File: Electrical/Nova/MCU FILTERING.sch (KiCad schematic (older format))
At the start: 13 parts

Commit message: Added Barometer, Flash, SD, and Power Supply
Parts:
- C? (x13): symbol Nova_Microcontroller:C -> Nova-rescue:C-Nova_Microcontroller
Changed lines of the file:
@@
 $Descr A4 11693 8268
 encoding utf-8
-Sheet 7 9
+Sheet 7 13
 Title "Microcontroller"
 Date "2020-07-02"
@@
 $EndBitmap
 $Comp
-L Nova_Microcontroller:C C?
+L Nova-rescue:C-Nova_Microcontroller C?
 U 1 1 5EEB15D0
 P 1600 3450
@@
 $EndComp
 $Comp
-L Nova_Microcontroller:C C?
+L Nova-rescue:C-Nova_Microcontroller C?
 U 1 1 5EEA7BC1
 P 2150 3450
@@
 $EndComp
 $Comp
-L Nova_Microcontroller:C C?
+L Nova-rescue:C-Nova_Microcontroller C?
 U 1 1 5EEA7EAA
 P 2650 3450
@@
 $EndComp
 $Comp
-L Nova_Microcontroller:C C?
+L Nova-rescue:C-Nova_Microcontroller C?
 U 1 1 5EEA8258
 P 3150 3450
@@
 $EndComp
 $Comp
-L Nova_Microcontroller:C C?
+L Nova-rescue:C-Nova_Microcontroller C?
 U 1 1 5EEA85B4
 P 3650 3450
@@
 $EndComp
 $Comp
-L Nova_Microcontroller:C C?
+L Nova-rescue:C-Nova_Microcontroller C?
 U 1 1 5EEA893A
 P 4150 3450
@@
 	3650 3000 4150 3000
 $Comp
-L Nova_Microcontroller:C C?
+L Nova-rescue:C-Nova_Microcontroller C?
 U 1 1 5EEADB63
 P 6350 3450
@@
 	6350 3300 6350 3100
 $Comp
-L Nova_Microcontroller:C C?
+L Nova-rescue:C-Nova_Microcontroller C?
 U 1 1 5EEAF36F
 P 4900 3450
@@
 $EndComp
 $Comp
-L Nova_Microcontroller:C C?
+L Nova-rescue:C-Nova_Microcontroller C?
 U 1 1 5EEAF915
 P 5450 3450
@@
 	5150 3100 5450 3100
 $Comp
-L Nova_Microcontroller:C C?
+L Nova-rescue:C-Nova_Microcontroller C?
 U 1 1 5EEB4CA7
 P 7350 3450
@@
 $EndComp
 $Comp
-L Nova_Microcontroller:C C?
+L Nova-rescue:C-Nova_Microcontroller C?
 U 1 1 5EEB51E9
 P 8000 3450
@@
 VREF CAPS
 $Comp
-L Nova_Microcontroller:C C?
+L Nova-rescue:C-Nova_Microcontroller C?
 U 1 1 5EEBBE66
 P 9450 3450
@@
 $EndComp
 $Comp
-L Nova_Microcontroller:C C?
+L Nova-rescue:C-Nova_Microcontroller C?
 U 1 1 5EEBC1C7
 P 10050 3450

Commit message: Fixed Power Supply
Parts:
- C? (x13): symbol Nova-rescue:C-Nova_Microcontroller -> Nova-rescue:C-Nova_Microcontroller-Nova-rescue
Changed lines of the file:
@@
 $EndBitmap
 $Comp
-L Nova-rescue:C-Nova_Microcontroller C?
+L Nova-rescue:C-Nova_Microcontroller-Nova-rescue C?
 U 1 1 5EEB15D0
 P 1600 3450
@@
 $EndComp
 $Comp
-L Nova-rescue:C-Nova_Microcontroller C?
+L Nova-rescue:C-Nova_Microcontroller-Nova-rescue C?
 U 1 1 5EEA7BC1
 P 2150 3450
@@
 $EndComp
 $Comp
-L Nova-rescue:C-Nova_Microcontroller C?
+L Nova-rescue:C-Nova_Microcontroller-Nova-rescue C?
 U 1 1 5EEA7EAA
 P 2650 3450
@@
 $EndComp
 $Comp
-L Nova-rescue:C-Nova_Microcontroller C?
+L Nova-rescue:C-Nova_Microcontroller-Nova-rescue C?
 U 1 1 5EEA8258
 P 3150 3450
@@
 $EndComp
 $Comp
-L Nova-rescue:C-Nova_Microcontroller C?
+L Nova-rescue:C-Nova_Microcontroller-Nova-rescue C?
 U 1 1 5EEA85B4
 P 3650 3450
@@
 $EndComp
 $Comp
-L Nova-rescue:C-Nova_Microcontroller C?
+L Nova-rescue:C-Nova_Microcontroller-Nova-rescue C?
 U 1 1 5EEA893A
 P 4150 3450
@@
 	3650 3000 4150 3000
 $Comp
-L Nova-rescue:C-Nova_Microcontroller C?
+L Nova-rescue:C-Nova_Microcontroller-Nova-rescue C?
 U 1 1 5EEADB63
 P 6350 3450
@@
 	6350 3300 6350 3100
 $Comp
-L Nova-rescue:C-Nova_Microcontroller C?
+L Nova-rescue:C-Nova_Microcontroller-Nova-rescue C?
 U 1 1 5EEAF36F
 P 4900 3450
@@
 $EndComp
 $Comp
-L Nova-rescue:C-Nova_Microcontroller C?
+L Nova-rescue:C-Nova_Microcontroller-Nova-rescue C?
 U 1 1 5EEAF915
 P 5450 3450
@@
 	5150 3100 5450 3100
 $Comp
-L Nova-rescue:C-Nova_Microcontroller C?
+L Nova-rescue:C-Nova_Microcontroller-Nova-rescue C?
 U 1 1 5EEB4CA7
 P 7350 3450
@@
 $EndComp
 $Comp
-L Nova-rescue:C-Nova_Microcontroller C?
+L Nova-rescue:C-Nova_Microcontroller-Nova-rescue C?
 U 1 1 5EEB51E9
 P 8000 3450
@@
 VREF CAPS
 $Comp
-L Nova-rescue:C-Nova_Microcontroller C?
+L Nova-rescue:C-Nova_Microcontroller-Nova-rescue C?
 U 1 1 5EEBBE66
 P 9450 3450
@@
 $EndComp
 $Comp
-L Nova-rescue:C-Nova_Microcontroller C?
+L Nova-rescue:C-Nova_Microcontroller-Nova-rescue C?
 U 1 1 5EEBC1C7
 P 10050 3450

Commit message: Added Gyroscope
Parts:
- C? (x13): symbol Nova-rescue:C-Nova_Microcontroller-Nova-rescue -> Nova-rescue:C-Nova_Microcontroller-Nova-rescue-Nova-rescue
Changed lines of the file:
@@
 $Descr A4 11693 8268
 encoding utf-8
-Sheet 7 13
+Sheet 7 14
 Title "Microcontroller"
 Date "2020-07-02"
@@
 $EndBitmap
 $Comp
-L Nova-rescue:C-Nova_Microcontroller-Nova-rescue C?
+L Nova-rescue:C-Nova_Microcontroller-Nova-rescue-Nova-rescue C?
 U 1 1 5EEB15D0
 P 1600 3450
@@
 $EndComp
 $Comp
-L Nova-rescue:C-Nova_Microcontroller-Nova-rescue C?
+L Nova-rescue:C-Nova_Microcontroller-Nova-rescue-Nova-rescue C?
 U 1 1 5EEA7BC1
 P 2150 3450
@@
 $EndComp
 $Comp
-L Nova-rescue:C-Nova_Microcontroller-Nova-rescue C?
+L Nova-rescue:C-Nova_Microcontroller-Nova-rescue-Nova-rescue C?
 U 1 1 5EEA7EAA
 P 2650 3450
@@
 $EndComp
 $Comp
-L Nova-rescue:C-Nova_Microcontroller-Nova-rescue C?
+L Nova-rescue:C-Nova_Microcontroller-Nova-rescue-Nova-rescue C?
 U 1 1 5EEA8258
 P 3150 3450
@@
 $EndComp
 $Comp
-L Nova-rescue:C-Nova_Microcontroller-Nova-rescue C?
+L Nova-rescue:C-Nova_Microcontroller-Nova-rescue-Nova-rescue C?
 U 1 1 5EEA85B4
 P 3650 3450
@@
 $EndComp
 $Comp
-L Nova-rescue:C-Nova_Microcontroller-Nova-rescue C?
+L Nova-rescue:C-Nova_Microcontroller-Nova-rescue-Nova-rescue C?
 U 1 1 5EEA893A
 P 4150 3450
@@
 	3650 3000 4150 3000
 $Comp
-L Nova-rescue:C-Nova_Microcontroller-Nova-rescue C?
+L Nova-rescue:C-Nova_Microcontroller-Nova-rescue-Nova-rescue C?
 U 1 1 5EEADB63
 P 6350 3450
@@
 	6350 3300 6350 3100
 $Comp
-L Nova-rescue:C-Nova_Microcontroller-Nova-rescue C?
+L Nova-rescue:C-Nova_Microcontroller-Nova-rescue-Nova-rescue C?
 U 1 1 5EEAF36F
 P 4900 3450
@@
 $EndComp
 $Comp
-L Nova-rescue:C-Nova_Microcontroller-Nova-rescue C?
+L Nova-rescue:C-Nova_Microcontroller-Nova-rescue-Nova-rescue C?
 U 1 1 5EEAF915
 P 5450 3450
@@
 	5150 3100 5450 3100
 $Comp
-L Nova-rescue:C-Nova_Microcontroller-Nova-rescue C?
+L Nova-rescue:C-Nova_Microcontroller-Nova-rescue-Nova-rescue C?
 U 1 1 5EEB4CA7
 P 7350 3450
@@
 $EndComp
 $Comp
-L Nova-rescue:C-Nova_Microcontroller-Nova-rescue C?
+L Nova-rescue:C-Nova_Microcontroller-Nova-rescue-Nova-rescue C?
 U 1 1 5EEB51E9
 P 8000 3450
@@
 VREF CAPS
 $Comp
-L Nova-rescue:C-Nova_Microcontroller-Nova-rescue C?
+L Nova-rescue:C-Nova_Microcontroller-Nova-rescue-Nova-rescue C?
 U 1 1 5EEBBE66
 P 9450 3450
@@
 $EndComp
 $Comp
-L Nova-rescue:C-Nova_Microcontroller-Nova-rescue C?
+L Nova-rescue:C-Nova_Microcontroller-Nova-rescue-Nova-rescue C?
 U 1 1 5EEBC1C7
 P 10050 3450

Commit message: Added Gyro pins. Organized Schematic
Need to determine if we need the interrupt pins for the sensors.
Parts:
- C? (x13): symbol Nova-rescue:C-Nova_Microcontroller-Nova-rescue-Nova-rescue -> Nova-rescue:C-Nova_Microcontroller-Nova-rescue-Nova-rescue-Nova-rescue
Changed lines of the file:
@@
 $EndBitmap
 $Comp
-L Nova-rescue:C-Nova_Microcontroller-Nova-rescue-Nova-rescue C?
+L Nova-rescue:C-Nova_Microcontroller-Nova-rescue-Nova-rescue-Nova-rescue C?
 U 1 1 5EEB15D0
 P 1600 3450
@@
 $EndComp
 $Comp
-L Nova-rescue:C-Nova_Microcontroller-Nova-rescue-Nova-rescue C?
+L Nova-rescue:C-Nova_Microcontroller-Nova-rescue-Nova-rescue-Nova-rescue C?
 U 1 1 5EEA7BC1
 P 2150 3450
@@
 $EndComp
 $Comp
-L Nova-rescue:C-Nova_Microcontroller-Nova-rescue-Nova-rescue C?
+L Nova-rescue:C-Nova_Microcontroller-Nova-rescue-Nova-rescue-Nova-rescue C?
 U 1 1 5EEA7EAA
 P 2650 3450
@@
 $EndComp
 $Comp
-L Nova-rescue:C-Nova_Microcontroller-Nova-rescue-Nova-rescue C?
+L Nova-rescue:C-Nova_Microcontroller-Nova-rescue-Nova-rescue-Nova-rescue C?
 U 1 1 5EEA8258
 P 3150 3450
@@
 $EndComp
 $Comp
-L Nova-rescue:C-Nova_Microcontroller-Nova-rescue-Nova-rescue C?
+L Nova-rescue:C-Nova_Microcontroller-Nova-rescue-Nova-rescue-Nova-rescue C?
 U 1 1 5EEA85B4
 P 3650 3450
@@
 $EndComp
 $Comp
-L Nova-rescue:C-Nova_Microcontroller-Nova-rescue-Nova-rescue C?
+L Nova-rescue:C-Nova_Microcontroller-Nova-rescue-Nova-rescue-Nova-rescue C?
 U 1 1 5EEA893A
 P 4150 3450
@@
 	3650 3000 4150 3000
 $Comp
-L Nova-rescue:C-Nova_Microcontroller-Nova-rescue-Nova-rescue C?
+L Nova-rescue:C-Nova_Microcontroller-Nova-rescue-Nova-rescue-Nova-rescue C?
 U 1 1 5EEADB63
 P 6350 3450
@@
 	6350 3300 6350 3100
 $Comp
-L Nova-rescue:C-Nova_Microcontroller-Nova-rescue-Nova-rescue C?
+L Nova-rescue:C-Nova_Microcontroller-Nova-rescue-Nova-rescue-Nova-rescue C?
 U 1 1 5EEAF36F
 P 4900 3450
@@
 $EndComp
 $Comp
-L Nova-rescue:C-Nova_Microcontroller-Nova-rescue-Nova-rescue C?
+L Nova-rescue:C-Nova_Microcontroller-Nova-rescue-Nova-rescue-Nova-rescue C?
 U 1 1 5EEAF915
 P 5450 3450
@@
 	5150 3100 5450 3100
 $Comp
-L Nova-rescue:C-Nova_Microcontroller-Nova-rescue-Nova-rescue C?
+L Nova-rescue:C-Nova_Microcontroller-Nova-rescue-Nova-rescue-Nova-rescue C?
 U 1 1 5EEB4CA7
 P 7350 3450
@@
 $EndComp
 $Comp
-L Nova-rescue:C-Nova_Microcontroller-Nova-rescue-Nova-rescue C?
+L Nova-rescue:C-Nova_Microcontroller-Nova-rescue-Nova-rescue-Nova-rescue C?
 U 1 1 5EEB51E9
 P 8000 3450
@@
 VREF CAPS
 $Comp
-L Nova-rescue:C-Nova_Microcontroller-Nova-rescue-Nova-rescue C?
+L Nova-rescue:C-Nova_Microcontroller-Nova-rescue-Nova-rescue-Nova-rescue C?
 U 1 1 5EEBBE66
 P 9450 3450
@@
 $EndComp
 $Comp
-L Nova-rescue:C-Nova_Microcontroller-Nova-rescue-Nova-rescue C?
+L Nova-rescue:C-Nova_Microcontroller-Nova-rescue-Nova-rescue-Nova-rescue C?
 U 1 1 5EEBC1C7
 P 10050 3450

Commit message: Added Pyro Channels
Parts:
- C? (x13): symbol Nova-rescue:C-Nova_Microcontroller-Nova-rescue-Nova-rescue-Nova-rescue -> Nova-rescue:C-Nova_Microcontroller-Nova-rescue-Nova-rescue-Nova-rescue-Nova-rescue
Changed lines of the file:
@@
 $Descr A4 11693 8268
 encoding utf-8
-Sheet 7 14
+Sheet 7 16
 Title "Microcontroller"
 Date "2020-07-02"
@@
 $EndBitmap
 $Comp
-L Nova-rescue:C-Nova_Microcontroller-Nova-rescue-Nova-rescue-Nova-rescue C?
+L Nova-rescue:C-Nova_Microcontroller-Nova-rescue-Nova-rescue-Nova-rescue-Nova-rescue C?
 U 1 1 5EEB15D0
 P 1600 3450
@@
 $EndComp
 $Comp
-L Nova-rescue:C-Nova_Microcontroller-Nova-rescue-Nova-rescue-Nova-rescue C?
+L Nova-rescue:C-Nova_Microcontroller-Nova-rescue-Nova-rescue-Nova-rescue-Nova-rescue C?
 U 1 1 5EEA7BC1
 P 2150 3450
@@
 $EndComp
 $Comp
-L Nova-rescue:C-Nova_Microcontroller-Nova-rescue-Nova-rescue-Nova-rescue C?
+L Nova-rescue:C-Nova_Microcontroller-Nova-rescue-Nova-rescue-Nova-rescue-Nova-rescue C?
 U 1 1 5EEA7EAA
 P 2650 3450
@@
 $EndComp
 $Comp
-L Nova-rescue:C-Nova_Microcontroller-Nova-rescue-Nova-rescue-Nova-rescue C?
+L Nova-rescue:C-Nova_Microcontroller-Nova-rescue-Nova-rescue-Nova-rescue-Nova-rescue C?
 U 1 1 5EEA8258
 P 3150 3450
@@
 $EndComp
 $Comp
-L Nova-rescue:C-Nova_Microcontroller-Nova-rescue-Nova-rescue-Nova-rescue C?
+L Nova-rescue:C-Nova_Microcontroller-Nova-rescue-Nova-rescue-Nova-rescue-Nova-rescue C?
 U 1 1 5EEA85B4
 P 3650 3450
@@
 $EndComp
 $Comp
-L Nova-rescue:C-Nova_Microcontroller-Nova-rescue-Nova-rescue-Nova-rescue C?
+L Nova-rescue:C-Nova_Microcontroller-Nova-rescue-Nova-rescue-Nova-rescue-Nova-rescue C?
 U 1 1 5EEA893A
 P 4150 3450
@@
 	3650 3000 4150 3000
 $Comp
-L Nova-rescue:C-Nova_Microcontroller-Nova-rescue-Nova-rescue-Nova-rescue C?
+L Nova-rescue:C-Nova_Microcontroller-Nova-rescue-Nova-rescue-Nova-rescue-Nova-rescue C?
 U 1 1 5EEADB63
 P 6350 3450
@@
 	6350 3300 6350 3100
 $Comp
-L Nova-rescue:C-Nova_Microcontroller-Nova-rescue-Nova-rescue-Nova-rescue C?
+L Nova-rescue:C-Nova_Microcontroller-Nova-rescue-Nova-rescue-Nova-rescue-Nova-rescue C?
 U 1 1 5EEAF36F
 P 4900 3450
@@
 $EndComp
 $Comp
-L Nova-rescue:C-Nova_Microcontroller-Nova-rescue-Nova-rescue-Nova-rescue C?
+L Nova-rescue:C-Nova_Microcontroller-Nova-rescue-Nova-rescue-Nova-rescue-Nova-rescue C?
 U 1 1 5EEAF915
 P 5450 3450
@@
 	5150 3100 5450 3100
 $Comp
-L Nova-rescue:C-Nova_Microcontroller-Nova-rescue-Nova-rescue-Nova-rescue C?
+L Nova-rescue:C-Nova_Microcontroller-Nova-rescue-Nova-rescue-Nova-rescue-Nova-rescue C?
 U 1 1 5EEB4CA7
 P 7350 3450
@@
 $EndComp
 $Comp
-L Nova-rescue:C-Nova_Microcontroller-Nova-rescue-Nova-rescue-Nova-rescue C?
+L Nova-rescue:C-Nova_Microcontroller-Nova-rescue-Nova-rescue-Nova-rescue-Nova-rescue C?
 U 1 1 5EEB51E9
 P 8000 3450
@@
 VREF CAPS
 $Comp
-L Nova-rescue:C-Nova_Microcontroller-Nova-rescue-Nova-rescue-Nova-rescue C?
+L Nova-rescue:C-Nova_Microcontroller-Nova-rescue-Nova-rescue-Nova-rescue-Nova-rescue C?
 U 1 1 5EEBBE66
 P 9450 3450
@@
 $EndComp
 $Comp
-L Nova-rescue:C-Nova_Microcontroller-Nova-rescue-Nova-rescue-Nova-rescue C?
+L Nova-rescue:C-Nova_Microcontroller-Nova-rescue-Nova-rescue-Nova-rescue-Nova-rescue C?
 U 1 1 5EEBC1C7
 P 10050 3450

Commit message: Added LED sheet and pins
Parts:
- C? (x13): symbol Nova-rescue:C-Nova_Microcontroller-Nova-rescue-Nova-rescue-Nova-rescue-Nova-rescue -> Nova-rescue:C-Nova_Microcontroller-Nova-rescue-Nova-rescue-Nova-rescue-Nova-rescue-Nova-rescue
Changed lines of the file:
@@
 $Descr A4 11693 8268
 encoding utf-8
-Sheet 7 16
+Sheet 7 18
 Title "Microcontroller"
 Date "2020-07-02"
@@
 $EndBitmap
 $Comp
-L Nova-rescue:C-Nova_Microcontroller-Nova-rescue-Nova-rescue-Nova-rescue-Nova-rescue C?
+L Nova-rescue:C-Nova_Microcontroller-Nova-rescue-Nova-rescue-Nova-rescue-Nova-rescue-Nova-rescue C?
 U 1 1 5EEB15D0
 P 1600 3450
@@
 $EndComp
 $Comp
-L Nova-rescue:C-Nova_Microcontroller-Nova-rescue-Nova-rescue-Nova-rescue-Nova-rescue C?
+L Nova-rescue:C-Nova_Microcontroller-Nova-rescue-Nova-rescue-Nova-rescue-Nova-rescue-Nova-rescue C?
 U 1 1 5EEA7BC1
 P 2150 3450
@@
 $EndComp
 $Comp
-L Nova-rescue:C-Nova_Microcontroller-Nova-rescue-Nova-rescue-Nova-rescue-Nova-rescue C?
+L Nova-rescue:C-Nova_Microcontroller-Nova-rescue-Nova-rescue-Nova-rescue-Nova-rescue-Nova-rescue C?
 U 1 1 5EEA7EAA
 P 2650 3450
@@
 $EndComp
 $Comp
-L Nova-rescue:C-Nova_Microcontroller-Nova-rescue-Nova-rescue-Nova-rescue-Nova-rescue C?
+L Nova-rescue:C-Nova_Microcontroller-Nova-rescue-Nova-rescue-Nova-rescue-Nova-rescue-Nova-rescue C?
 U 1 1 5EEA8258
 P 3150 3450
@@
 $EndComp
 $Comp
-L Nova-rescue:C-Nova_Microcontroller-Nova-rescue-Nova-rescue-Nova-rescue-Nova-rescue C?
+L Nova-rescue:C-Nova_Microcontroller-Nova-rescue-Nova-rescue-Nova-rescue-Nova-rescue-Nova-rescue C?
 U 1 1 5EEA85B4
 P 3650 3450
@@
 $EndComp
 $Comp
-L Nova-rescue:C-Nova_Microcontroller-Nova-rescue-Nova-rescue-Nova-rescue-Nova-rescue C?
+L Nova-rescue:C-Nova_Microcontroller-Nova-rescue-Nova-rescue-Nova-rescue-Nova-rescue-Nova-rescue C?
 U 1 1 5EEA893A
 P 4150 3450
@@
 	3650 3000 4150 3000
 $Comp
-L Nova-rescue:C-Nova_Microcontroller-Nova-rescue-Nova-rescue-Nova-rescue-Nova-rescue C?
+L Nova-rescue:C-Nova_Microcontroller-Nova-rescue-Nova-rescue-Nova-rescue-Nova-rescue-Nova-rescue C?
 U 1 1 5EEADB63
 P 6350 3450
@@
 	6350 3300 6350 3100
 $Comp
-L Nova-rescue:C-Nova_Microcontroller-Nova-rescue-Nova-rescue-Nova-rescue-Nova-rescue C?
+L Nova-rescue:C-Nova_Microcontroller-Nova-rescue-Nova-rescue-Nova-rescue-Nova-rescue-Nova-rescue C?
 U 1 1 5EEAF36F
 P 4900 3450
@@
 $EndComp
 $Comp
-L Nova-rescue:C-Nova_Microcontroller-Nova-rescue-Nova-rescue-Nova-rescue-Nova-rescue C?
+L Nova-rescue:C-Nova_Microcontroller-Nova-rescue-Nova-rescue-Nova-rescue-Nova-rescue-Nova-rescue C?
 U 1 1 5EEAF915
 P 5450 3450
@@
 	5150 3100 5450 3100
 $Comp
-L Nova-rescue:C-Nova_Microcontroller-Nova-rescue-Nova-rescue-Nova-rescue-Nova-rescue C?
+L Nova-rescue:C-Nova_Microcontroller-Nova-rescue-Nova-rescue-Nova-rescue-Nova-rescue-Nova-rescue C?
 U 1 1 5EEB4CA7
 P 7350 3450
@@
 $EndComp
 $Comp
-L Nova-rescue:C-Nova_Microcontroller-Nova-rescue-Nova-rescue-Nova-rescue-Nova-rescue C?
+L Nova-rescue:C-Nova_Microcontroller-Nova-rescue-Nova-rescue-Nova-rescue-Nova-rescue-Nova-rescue C?
 U 1 1 5EEB51E9
 P 8000 3450
@@
 VREF CAPS
 $Comp
-L Nova-rescue:C-Nova_Microcontroller-Nova-rescue-Nova-rescue-Nova-rescue-Nova-rescue C?
+L Nova-rescue:C-Nova_Microcontroller-Nova-rescue-Nova-rescue-Nova-rescue-Nova-rescue-Nova-rescue C?
 U 1 1 5EEBBE66
 P 9450 3450
@@
 $EndComp
 $Comp
-L Nova-rescue:C-Nova_Microcontroller-Nova-rescue-Nova-rescue-Nova-rescue-Nova-rescue C?
+L Nova-rescue:C-Nova_Microcontroller-Nova-rescue-Nova-rescue-Nova-rescue-Nova-rescue-Nova-rescue C?
 U 1 1 5EEBC1C7
 P 10050 3450

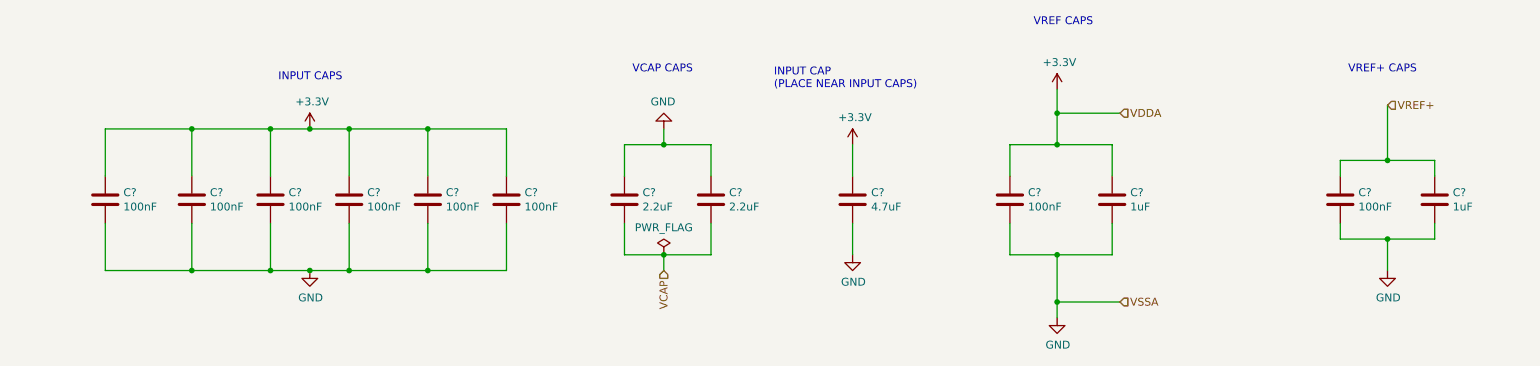
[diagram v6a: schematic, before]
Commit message: Minor update
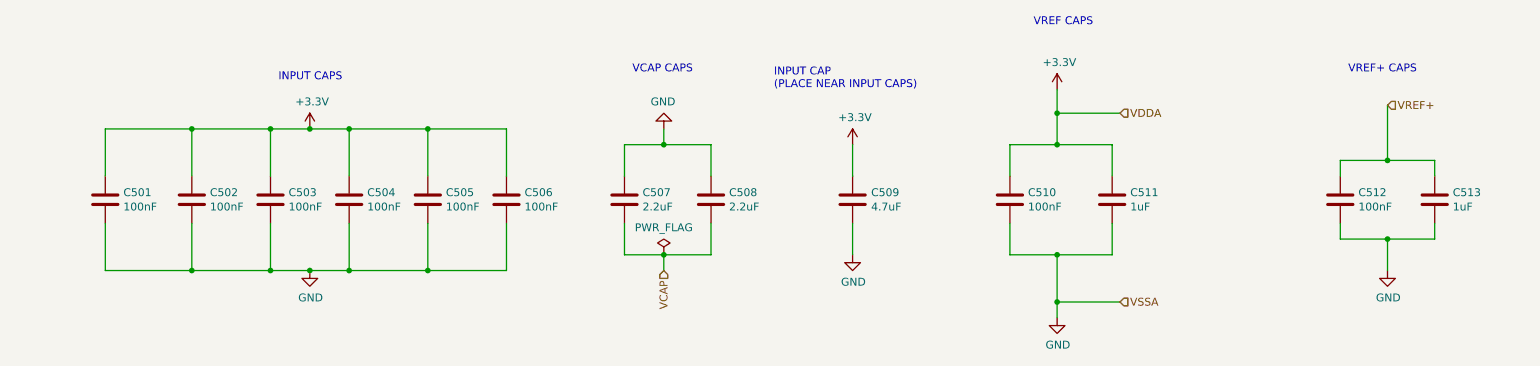
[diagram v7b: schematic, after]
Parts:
- C501, C502, C503, C504, C505, C506, C507, C508, C509, C510, C511, C512, C513: renamed from C?; footprint NOVA MCU (STM):C_0805_2012Metric_Pad1.15x1.40mm_HandSolder -> NOVA MCU (STM):C_0805_2012Metric

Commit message: Added Accelerometer
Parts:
- C501, C502, C503, C504, C505, C506, C507, C508, C509, C510, C511, C512, C513: symbol Nova-rescue:C-Nova_Microcontroller-Nova-rescue-Nova-rescue-Nova-rescue-Nova-rescue-Nova-rescue -> Nova-rescue:C-Nova_Microcontroller-Nova-rescue-Nova-rescue-Nova-rescue-Nova-rescue-Nova-rescue-Nova-rescue
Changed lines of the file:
@@
 $Descr A4 11693 8268
 encoding utf-8
-Sheet 5 18
+Sheet 5 19
 Title "Microcontroller"
 Date "2020-07-02"
@@
 $EndBitmap
 $Comp
-L Nova-rescue:C-Nova_Microcontroller-Nova-rescue-Nova-rescue-Nova-rescue-Nova-rescue-Nova-rescue C501
+L Nova-rescue:C-Nova_Microcontroller-Nova-rescue-Nova-rescue-Nova-rescue-Nova-rescue-Nova-rescue-Nova-rescue C501
 U 1 1 5EEB15D0
 P 1600 3450
@@
 $EndComp
 $Comp
-L Nova-rescue:C-Nova_Microcontroller-Nova-rescue-Nova-rescue-Nova-rescue-Nova-rescue-Nova-rescue C502
+L Nova-rescue:C-Nova_Microcontroller-Nova-rescue-Nova-rescue-Nova-rescue-Nova-rescue-Nova-rescue-Nova-rescue C502
 U 1 1 5EEA7BC1
 P 2150 3450
@@
 $EndComp
 $Comp
-L Nova-rescue:C-Nova_Microcontroller-Nova-rescue-Nova-rescue-Nova-rescue-Nova-rescue-Nova-rescue C503
+L Nova-rescue:C-Nova_Microcontroller-Nova-rescue-Nova-rescue-Nova-rescue-Nova-rescue-Nova-rescue-Nova-rescue C503
 U 1 1 5EEA7EAA
 P 2650 3450
@@
 $EndComp
 $Comp
-L Nova-rescue:C-Nova_Microcontroller-Nova-rescue-Nova-rescue-Nova-rescue-Nova-rescue-Nova-rescue C504
+L Nova-rescue:C-Nova_Microcontroller-Nova-rescue-Nova-rescue-Nova-rescue-Nova-rescue-Nova-rescue-Nova-rescue C504
 U 1 1 5EEA8258
 P 3150 3450
@@
 $EndComp
 $Comp
-L Nova-rescue:C-Nova_Microcontroller-Nova-rescue-Nova-rescue-Nova-rescue-Nova-rescue-Nova-rescue C505
+L Nova-rescue:C-Nova_Microcontroller-Nova-rescue-Nova-rescue-Nova-rescue-Nova-rescue-Nova-rescue-Nova-rescue C505
 U 1 1 5EEA85B4
 P 3650 3450
@@
 $EndComp
 $Comp
-L Nova-rescue:C-Nova_Microcontroller-Nova-rescue-Nova-rescue-Nova-rescue-Nova-rescue-Nova-rescue C506
+L Nova-rescue:C-Nova_Microcontroller-Nova-rescue-Nova-rescue-Nova-rescue-Nova-rescue-Nova-rescue-Nova-rescue C506
 U 1 1 5EEA893A
 P 4150 3450
@@
 	3650 3000 4150 3000
 $Comp
-L Nova-rescue:C-Nova_Microcontroller-Nova-rescue-Nova-rescue-Nova-rescue-Nova-rescue-Nova-rescue C509
+L Nova-rescue:C-Nova_Microcontroller-Nova-rescue-Nova-rescue-Nova-rescue-Nova-rescue-Nova-rescue-Nova-rescue C509
 U 1 1 5EEADB63
 P 6350 3450
@@
 	6350 3300 6350 3100
 $Comp
-L Nova-rescue:C-Nova_Microcontroller-Nova-rescue-Nova-rescue-Nova-rescue-Nova-rescue-Nova-rescue C507
+L Nova-rescue:C-Nova_Microcontroller-Nova-rescue-Nova-rescue-Nova-rescue-Nova-rescue-Nova-rescue-Nova-rescue C507
 U 1 1 5EEAF36F
 P 4900 3450
@@
 $EndComp
 $Comp
-L Nova-rescue:C-Nova_Microcontroller-Nova-rescue-Nova-rescue-Nova-rescue-Nova-rescue-Nova-rescue C508
+L Nova-rescue:C-Nova_Microcontroller-Nova-rescue-Nova-rescue-Nova-rescue-Nova-rescue-Nova-rescue-Nova-rescue C508
 U 1 1 5EEAF915
 P 5450 3450
@@
 	5150 3100 5450 3100
 $Comp
-L Nova-rescue:C-Nova_Microcontroller-Nova-rescue-Nova-rescue-Nova-rescue-Nova-rescue-Nova-rescue C510
+L Nova-rescue:C-Nova_Microcontroller-Nova-rescue-Nova-rescue-Nova-rescue-Nova-rescue-Nova-rescue-Nova-rescue C510
 U 1 1 5EEB4CA7
 P 7350 3450
@@
 $EndComp
 $Comp
-L Nova-rescue:C-Nova_Microcontroller-Nova-rescue-Nova-rescue-Nova-rescue-Nova-rescue-Nova-rescue C511
+L Nova-rescue:C-Nova_Microcontroller-Nova-rescue-Nova-rescue-Nova-rescue-Nova-rescue-Nova-rescue-Nova-rescue C511
 U 1 1 5EEB51E9
 P 8000 3450
@@
 VREF CAPS
 $Comp
-L Nova-rescue:C-Nova_Microcontroller-Nova-rescue-Nova-rescue-Nova-rescue-Nova-rescue-Nova-rescue C512
+L Nova-rescue:C-Nova_Microcontroller-Nova-rescue-Nova-rescue-Nova-rescue-Nova-rescue-Nova-rescue-Nova-rescue C512
 U 1 1 5EEBBE66
 P 9450 3450
@@
 $EndComp
 $Comp
-L Nova-rescue:C-Nova_Microcontroller-Nova-rescue-Nova-rescue-Nova-rescue-Nova-rescue-Nova-rescue C513
+L Nova-rescue:C-Nova_Microcontroller-Nova-rescue-Nova-rescue-Nova-rescue-Nova-rescue-Nova-rescue-Nova-rescue C513
 U 1 1 5EEBC1C7
 P 10050 3450
